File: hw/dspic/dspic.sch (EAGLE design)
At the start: 25 parts, among them Q1 8MHz, U1 DSPIC33FJ128MC802-I/SP

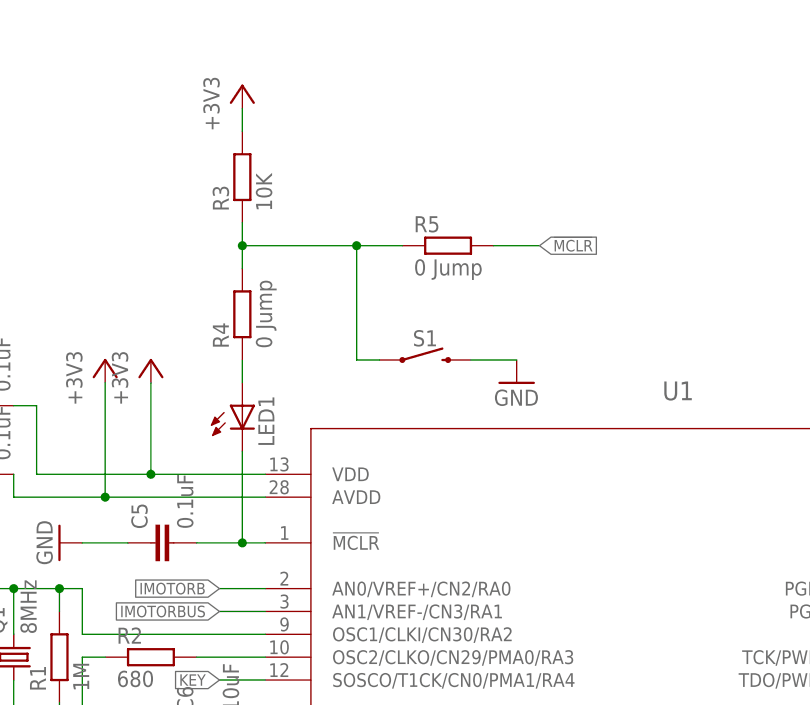
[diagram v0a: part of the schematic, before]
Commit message: config
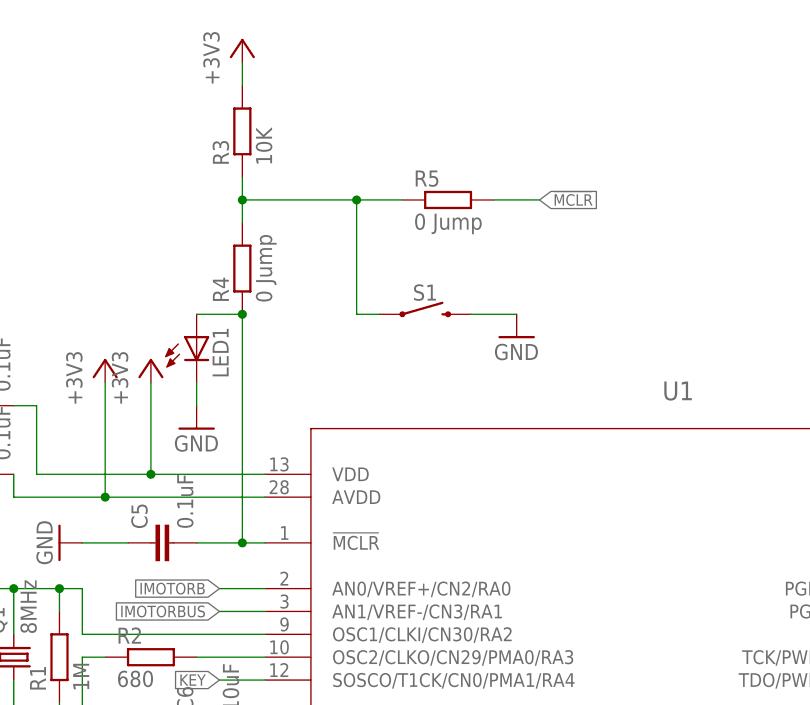
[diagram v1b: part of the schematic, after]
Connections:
- removed net N$5: LED1.A, R4.1
- net GND: now also LED1.C
- net N$2: now also LED1.A, R4.1; no longer LED1.C
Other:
- moved on the sheet: LED1, R3, R4, R5, S1
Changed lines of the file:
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@@
 <part name="J2" library="SparkFun-Connectors" deviceset="CONN_02" device=""/>
 <part name="SV4" library="con-lstb" deviceset="MA05-1" device=""/>
+<part name="GND11" library="supply1" deviceset="GND" device=""/>
 </parts>
 <sheets>
@@
 </plain>
 <instances>
-<instance part="R3" gate="G$1" x="40.64" y="114.3" rot="R90"/>
+<instance part="R3" gate="G$1" x="40.64" y="119.38" rot="R90"/>
 <instance part="C6" gate="G$1" x="35.56" y="53.34" rot="R90"/>
 <instance part="GND5" gate="1" x="30.48" y="40.64"/>
@@
 <instance part="GND2" gate="1" x="2.54" y="88.9" rot="R270"/>
 <instance part="+3V32" gate="G$1" x="30.48" y="93.98"/>
-<instance part="+3V33" gate="G$1" x="40.64" y="124.46"/>
+<instance part="+3V33" gate="G$1" x="40.64" y="129.54"/>
 <instance part="C5" gate="G$1" x="30.48" y="73.66" rot="R90"/>
 <instance part="GND4" gate="1" x="20.32" y="73.66" rot="R270"/>
-<instance part="S1" gate="G$1" x="60.96" y="93.98"/>
-<instance part="GND6" gate="1" x="71.12" y="91.44"/>
+<instance part="S1" gate="G$1" x="60.96" y="99.06"/>
+<instance part="GND6" gate="1" x="71.12" y="96.52"/>
 <instance part="+3V35" gate="G$1" x="170.18" y="81.28"/>
 <instance part="GND9" gate="1" x="170.18" y="71.12" rot="R270"/>
@@
 <instance part="SV3" gate="G$1" x="182.88" y="17.78" rot="R180"/>
 <instance part="GND8" gate="1" x="165.1" y="7.62"/>
-<instance part="LED1" gate="G$1" x="40.64" y="88.9"/>
+<instance part="LED1" gate="G$1" x="35.56" y="96.52"/>
 <instance part="S2" gate="G$1" x="195.58" y="93.98"/>
 <instance part="+3V36" gate="G$1" x="203.2" y="101.6"/>
@@
 <instance part="R1" gate="G$1" x="20.32" y="60.96" rot="R90"/>
 <instance part="SV1" gate="G$1" x="165.1" y="60.96" rot="R180"/>
-<instance part="R4" gate="G$1" x="40.64" y="99.06" rot="R90"/>
-<instance part="R5" gate="G$1" x="63.5" y="106.68"/>
+<instance part="R4" gate="G$1" x="40.64" y="104.14" rot="R90"/>
+<instance part="R5" gate="G$1" x="63.5" y="111.76"/>
 <instance part="R6" gate="G$1" x="152.4" y="93.98"/>
 <instance part="J2" gate="G$1" x="154.94" y="76.2" rot="R180"/>
 <instance part="SV4" gate="G$1" x="193.04" y="71.12" rot="R180"/>
+<instance part="GND11" gate="1" x="35.56" y="86.36"/>
 </instances>
 <busses>
@@
 <pinref part="S1" gate="G$1" pin="2"/>
 <pinref part="GND6" gate="1" pin="GND"/>
-<wire x1="66.04" y1="93.98" x2="71.12" y2="93.98" width="0.1524" layer="91"/>
+<wire x1="66.04" y1="99.06" x2="71.12" y2="99.06" width="0.1524" layer="91"/>
 </segment>
 <segment>
@@
 <wire x1="129.54" y1="20.32" x2="129.54" y2="17.78" width="0.1524" layer="91"/>
 </segment>
+<segment>
+<pinref part="GND11" gate="1" pin="GND"/>
+<pinref part="LED1" gate="G$1" pin="C"/>
+<wire x1="35.56" y1="88.9" x2="35.56" y2="91.44" width="0.1524" layer="91"/>
+</segment>
 </net>
 <net name="+3V3" class="0">
@@
 <pinref part="R3" gate="G$1" pin="2"/>
 <pinref part="+3V33" gate="G$1" pin="+3V3"/>
-<wire x1="40.64" y1="119.38" x2="40.64" y2="121.92" width="0.1524" layer="91"/>
+<wire x1="40.64" y1="124.46" x2="40.64" y2="127" width="0.1524" layer="91"/>
 </segment>
 <segment>
@@
 <segment>
 <pinref part="R5" gate="G$1" pin="2"/>
-<wire x1="68.58" y1="106.68" x2="73.66" y2="106.68" width="0.1524" layer="91"/>
-<label x="73.66" y="106.68" size="1.27" layer="95" xref="yes"/>
+<wire x1="68.58" y1="111.76" x2="73.66" y2="111.76" width="0.1524" layer="91"/>
+<label x="73.66" y="111.76" size="1.27" layer="95" xref="yes"/>
 </segment>
 </net>
@@
 <segment>
 <wire x1="43.18" y1="73.66" x2="40.64" y2="73.66" width="0.1524" layer="91"/>
+<pinref part="U1" gate="&gt;NAME" pin="!MCLR!"/>
+<pinref part="LED1" gate="G$1" pin="A"/>
+<pinref part="R4" gate="G$1" pin="1"/>
+<wire x1="35.56" y1="99.06" x2="40.64" y2="99.06" width="0.1524" layer="91"/>
+<wire x1="40.64" y1="73.66" x2="40.64" y2="99.06" width="0.1524" layer="91"/>
+<junction x="40.64" y="99.06"/>
 <pinref part="C5" gate="G$1" pin="2"/>
-<pinref part="LED1" gate="G$1" pin="C"/>
-<wire x1="40.64" y1="73.66" x2="35.56" y2="73.66" width="0.1524" layer="91"/>
-<wire x1="40.64" y1="83.82" x2="40.64" y2="73.66" width="0.1524" layer="91"/>
+<wire x1="35.56" y1="73.66" x2="40.64" y2="73.66" width="0.1524" layer="91"/>
 <junction x="40.64" y="73.66"/>
-<pinref part="U1" gate="&gt;NAME" pin="!MCLR!"/>
 </segment>
 </net>
@@
 </segment>
 </net>
-<net name="N$5" class="0">
-<segment>
-<pinref part="LED1" gate="G$1" pin="A"/>
-<pinref part="R4" gate="G$1" pin="1"/>
-<wire x1="40.64" y1="91.44" x2="40.64" y2="93.98" width="0.1524" layer="91"/>
-</segment>
-</net>
 <net name="N$4" class="0">
 <segment>
 <pinref part="R3" gate="G$1" pin="1"/>
 <pinref part="R4" gate="G$1" pin="2"/>
-<wire x1="40.64" y1="109.22" x2="40.64" y2="106.68" width="0.1524" layer="91"/>
+<wire x1="40.64" y1="114.3" x2="40.64" y2="111.76" width="0.1524" layer="91"/>
 <pinref part="R5" gate="G$1" pin="1"/>
-<wire x1="40.64" y1="106.68" x2="40.64" y2="104.14" width="0.1524" layer="91"/>
-<wire x1="58.42" y1="106.68" x2="53.34" y2="106.68" width="0.1524" layer="91"/>
-<junction x="40.64" y="106.68"/>
+<wire x1="40.64" y1="111.76" x2="40.64" y2="109.22" width="0.1524" layer="91"/>
+<wire x1="58.42" y1="111.76" x2="53.34" y2="111.76" width="0.1524" layer="91"/>
+<junction x="40.64" y="111.76"/>
 <pinref part="S1" gate="G$1" pin="1"/>
-<wire x1="53.34" y1="106.68" x2="40.64" y2="106.68" width="0.1524" layer="91"/>
-<wire x1="55.88" y1="93.98" x2="53.34" y2="93.98" width="0.1524" layer="91"/>
-<wire x1="53.34" y1="93.98" x2="53.34" y2="106.68" width="0.1524" layer="91"/>
-<junction x="53.34" y="106.68"/>
-</segment>
-</net>
+<wire x1="53.34" y1="111.76" x2="40.64" y2="111.76" width="0.1524" layer="91"/>
+<wire x1="55.88" y1="99.06" x2="53.34" y2="99.06" width="0.1524" layer="91"/>
+<wire x1="53.34" y1="99.06" x2="53.34" y2="111.76" width="0.1524" layer="91"/>
+<junction x="53.34" y="111.76"/>
+</segment>
+</net>
